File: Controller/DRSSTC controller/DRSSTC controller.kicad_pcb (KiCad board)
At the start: 2 copper layers, 110.5 x 47 mm, 108 parts, among them J1 Conn_01x01_Female, J2 Screw_Terminal_01x02, J3 Conn_01x01_Female, J4 Conn_01x01_Female, J401 Conn_01x01_Female, J402 Screw_Terminal_01x02, J403 Conn_01x01_Female, J5 Screw_Terminal_01x02, J507 Conn_01x03_Male, J508 Conn_01x02_Male, J509 Conn_01x02_Male, J510 Conn_01x02_Male, J6 Conn_01x01_Female, J7 Conn_01x01_Female, J8 Screw_Terminal_01x02, J9 Conn_01x01_Female, Q401 Q_PMOS_GDS, Q402 Q_NMOS_GDS, Q403 Q_PMOS_GDS, Q404 Q_NMOS_GDS, U401 UCC27524, U501 Optical_reciver, U502 Optical_reciver, U503 74HC14, U504 LM311, U505 74HC74, U506 74LS00, U507 TLV7031DBV, U601 L7809, U602 L7805

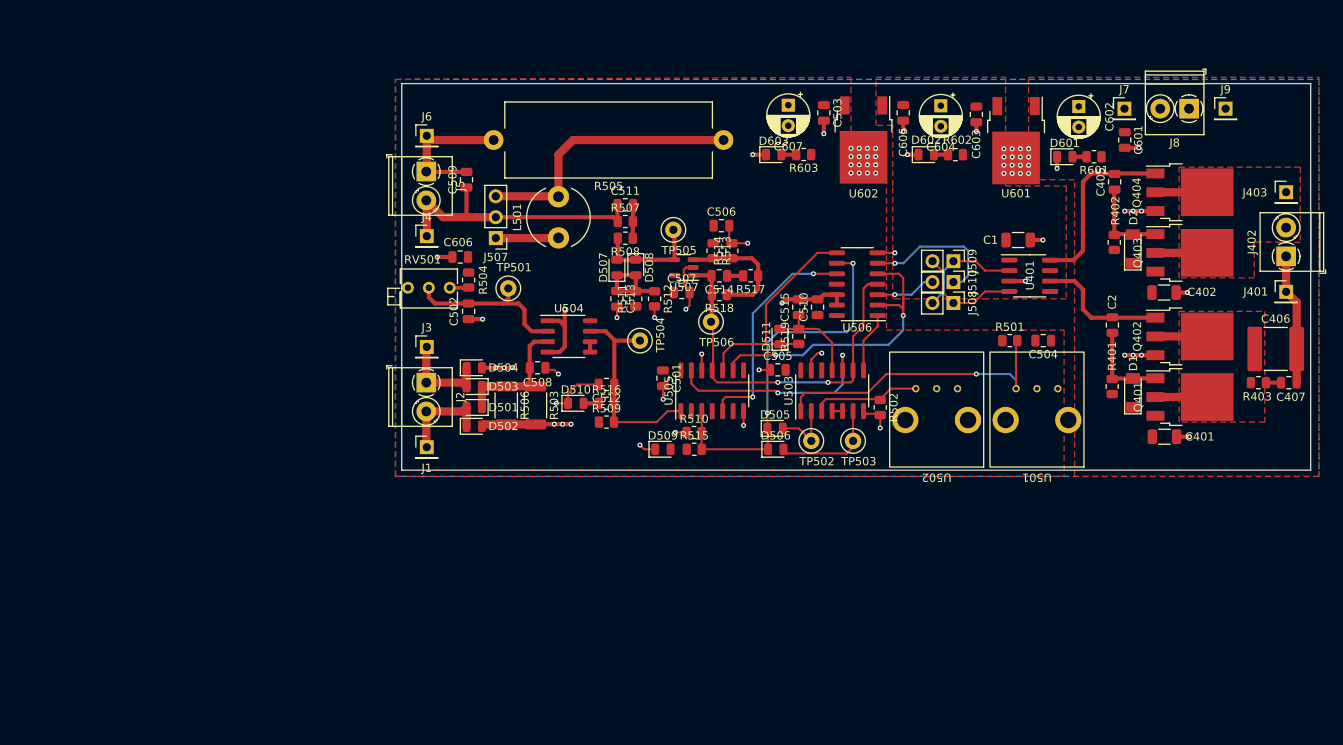
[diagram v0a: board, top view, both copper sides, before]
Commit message: V0.15a
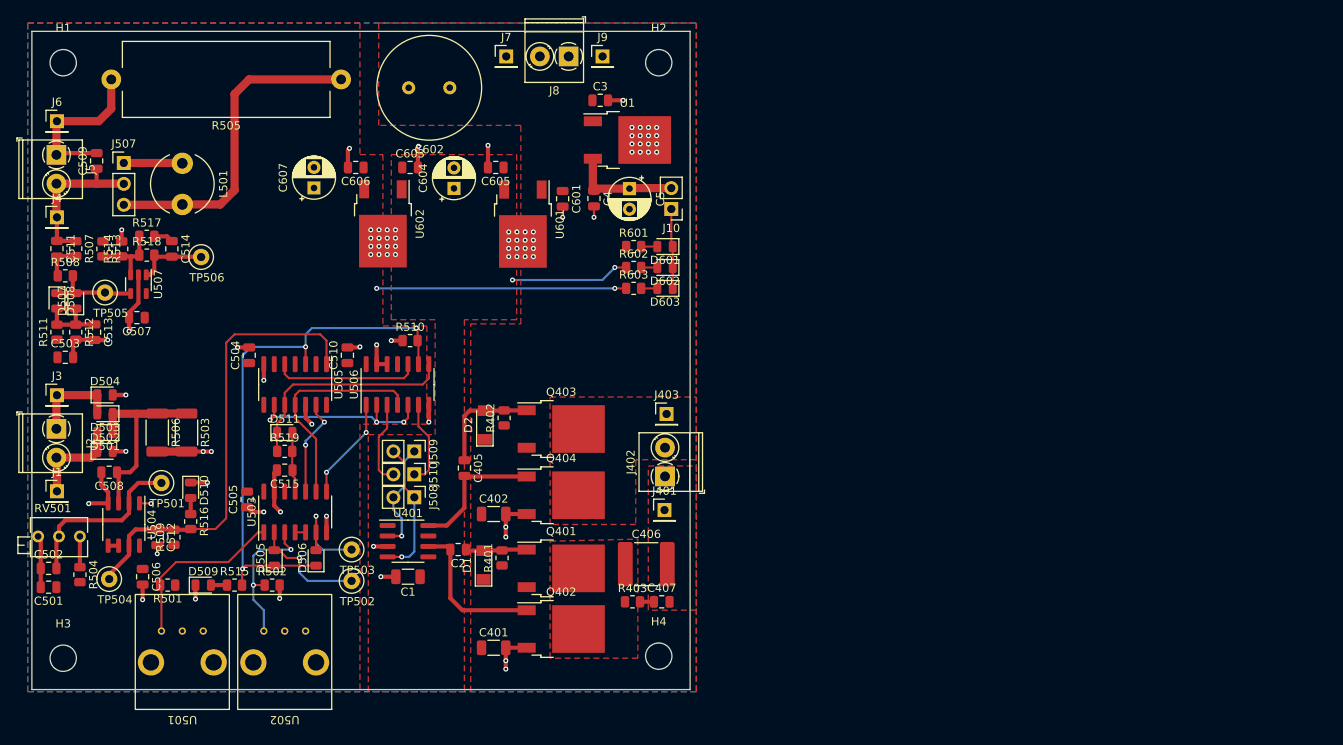
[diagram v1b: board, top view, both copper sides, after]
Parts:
- added C3: 100n, Capacitor_SMD:C_0805_2012Metric, F.Cu at (115.3, 90.7)
- added C4: 100n, Capacitor_SMD:C_0805_2012Metric, F.Cu at (114.6, 102.6)
- added C5: 470u, Capacitor_THT:CP_Radial_D5.0mm_P2.50mm, F.Cu at (118.9, 101.4)
- added H1: MountingHole, MountingHole:MountingHole_3.2mm_M3, F.Cu at (50.0, 86.1)
- added H2: MountingHole, MountingHole:MountingHole_3.2mm_M3, F.Cu at (122.4, 86.1)
- added H3: MountingHole, MountingHole:MountingHole_3.2mm_M3, F.Cu at (50.0, 158.5)
- added H4: MountingHole, MountingHole:MountingHole_3.2mm_M3, F.Cu at (122.4, 158.2)
- added J10: Conn_01x02_Male, Connector_PinHeader_2.54mm:PinHeader_1x02_P2.54mm_Vertical, F.Cu at (124.0, 103.9)
- added U1: L7812, Package_TO_SOT_SMD:TO-252-2, F.Cu at (118.6, 95.5)
- C602: footprint Capacitor_THT:CP_Radial_D5.0mm_P2.50mm -> Capacitor_THT:C_Radial_D12.5mm_H25.0mm_P5.00mm
- Q401, Q402, Q403, Q404: footprint Package_TO_SOT_SMD:TO-252-3_TabPin2 -> Package_TO_SOT_SMD:TO-252-2
- moved U501 108.0 mm to (64.5, 155.2)
- moved R501 106.6 mm to (62.7, 149.6), turned to 180 degrees
- moved C503 96.9 mm to (50.3, 121.9), turned to 0 degrees
- moved C504 96.5 mm to (72.6, 121.7), turned to 90 degrees
- moved C405 86.4 mm to (98.8, 135.4), turned to -90 degrees
- moved C402 85.8 mm to (102.4, 141.0)
- moved C401 85.5 mm to (102.4, 157.2)
- moved Q404 84.8 mm to (110.6, 138.7)
- moved C1 84.7 mm to (91.9, 148.6), turned to 180 degrees
- moved U502 84.5 mm to (77.0, 155.2)
- moved Q402 84.3 mm to (110.6, 154.9)
- moved C2 84.1 mm to (98.0, 145.3), turned to 180 degrees
- moved C506 82.3 mm to (59.7, 148.6), turned to -90 degrees
- moved U401 82.2 mm to (91.9, 144.3)
- moved D1 81.7 mm to (101.1, 147.2)
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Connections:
- net Net-(C405-Pad1) renamed /GDT_primary/BottomSide_PGate
- net Net-(C405-Pad2) renamed /GDT_primary/BottomSide_NGate
- net Net-(C406-Pad2) renamed /GDT_primary/GDT_terminal_B
- net Net-(D601-Pad2) renamed /Power_regulation/Vcc_LED
- net Net-(D602-Pad2) renamed /Power_regulation/9V_LED
- net Net-(D603-Pad2) renamed /Power_regulation/5V_LED
- net Net-(J402-Pad2) renamed /GDT_primary/GDT_terminal_A
- net Net-(Q401-Pad1) renamed /GDT_primary/TopSide_PGate
- net Net-(Q402-Pad1) renamed /GDT_primary/TopSide_NGate
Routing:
- net LED_overcurrent: track 25.5 -> 56.1 mm
- net +5V: track 0.00 -> 30.3 mm, vias 0 -> 2
- net LED_inteep: track 47.2 -> 67.1 mm, vias 2 -> 3
- net /GDT_primary/GDT_terminal_B: track 15.9 -> 0.00 mm
- net Net-(C509-Pad1): track 34.5 -> 19.3 mm
- net Net-(R501-Pad2): track 36.4 -> 21.4 mm, vias 1 -> 0
- net Net-(U505-Pad9): track 37.8 -> 23.1 mm, vias 2 -> 3
- net +9V: track 0.00 -> 14.5 mm, vias 0 -> 2
- net Net-(U503-Pad10): track 26.3 -> 11.9 mm
- net +12V: track 0.00 -> 13.5 mm
- net Net-(C406-Pad1): track 12.6 -> 0.00 mm
- net /GDT_primary/GDT_terminal_A: track 12.6 -> 0.00 mm
- net Net-(C514-Pad2): track 45.8 -> 35.7 mm, vias 2 -> 0
- net Net-(U505-Pad5): track 27.5 -> 17.8 mm, vias 2 -> 0
- net GND: track 100.3 -> 107.9 mm, vias 74 -> 84
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- added copper zone on F.Cu, net /GDT_primary/GDT_terminal_B
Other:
- board size 110.5 x 47 mm -> 80 x 80 mm
